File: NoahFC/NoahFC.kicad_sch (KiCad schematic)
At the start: 30 parts, among them J1 ALERON, J10 GND, J11 SCK, J12 MISO, J13 VCC, J14 GND, J2 ELEVATOR, J3 MPU6050, J4 FTDI, J5 VCC, J6 THROTTLE, J7 PPM, J8 GPS, U1 ATmega328, U3 AMS1117-5.0, Y1 16Mhz

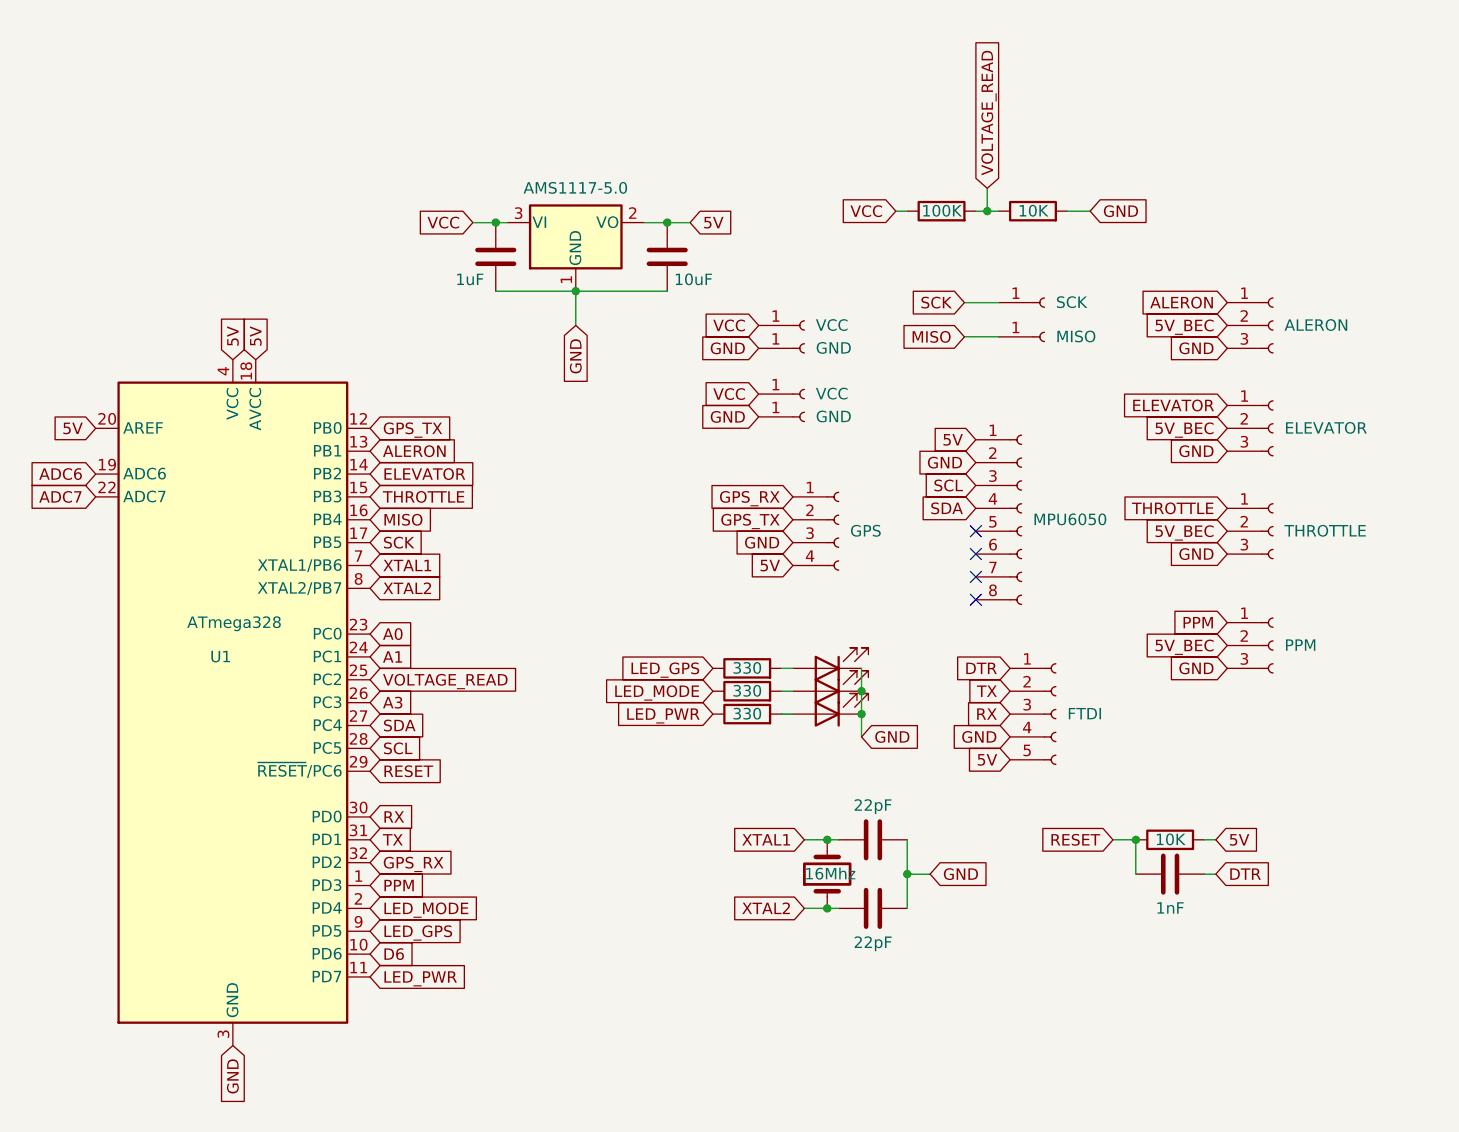
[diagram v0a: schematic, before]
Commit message: route board
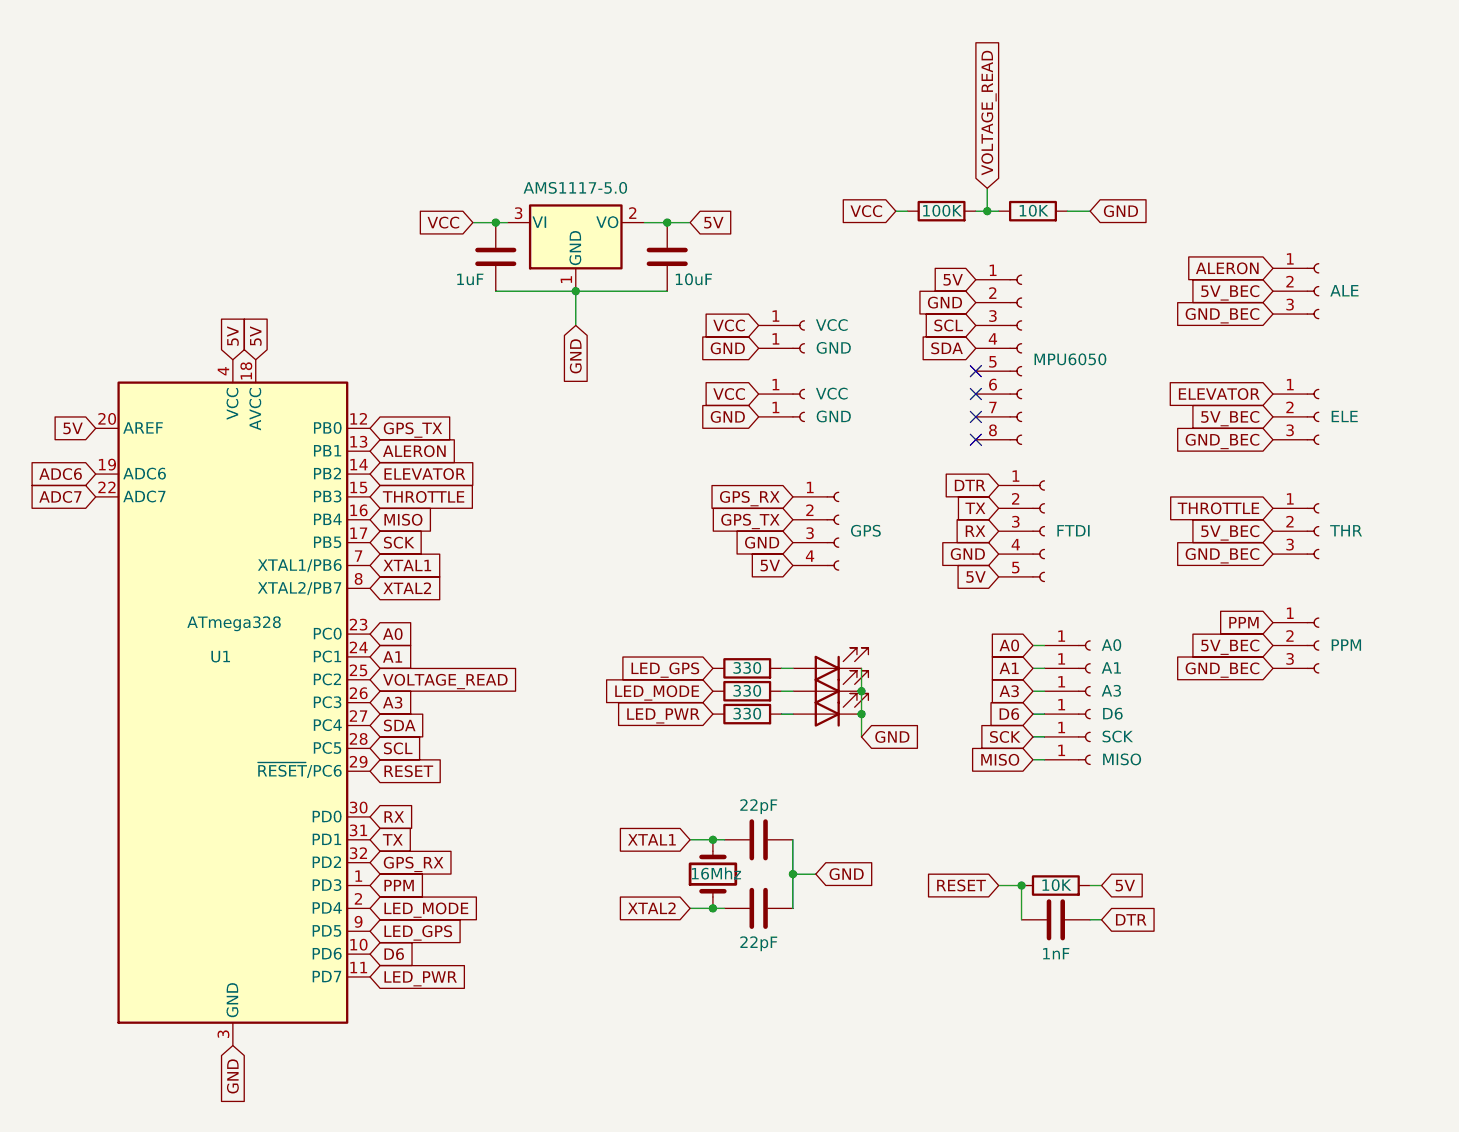
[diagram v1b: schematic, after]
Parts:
- added J15: A1, TestPoint:TestPoint_Pad_1.0x1.0mm, symbol Connector:Conn_01x01_Female
- added J16: A3, TestPoint:TestPoint_Pad_1.0x1.0mm, symbol Connector:Conn_01x01_Female
- added J17: D6, TestPoint:TestPoint_Pad_1.0x1.0mm, symbol Connector:Conn_01x01_Female
- added J9: A0, TestPoint:TestPoint_Pad_1.0x1.0mm, symbol Connector:Conn_01x01_Female
- J1: value ALERON -> ALE
- J2: value ELEVATOR -> ELE
- J6: value THROTTLE -> THR
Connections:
- net A0: now also J9.1 (Pin_1)
- net A1: now also J15.1 (Pin_1)
- net A3: now also J16.1 (Pin_1)
- net D6: now also J17.1 (Pin_1)
- net GND: no longer J1.3 (Pin_3), J2.3 (Pin_3), J6.3 (Pin_3), J7.3 (Pin_3)
- new net GND_BEC: J1.3 (Pin_3), J2.3 (Pin_3), J6.3 (Pin_3), J7.3 (Pin_3)

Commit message: rev1 updates
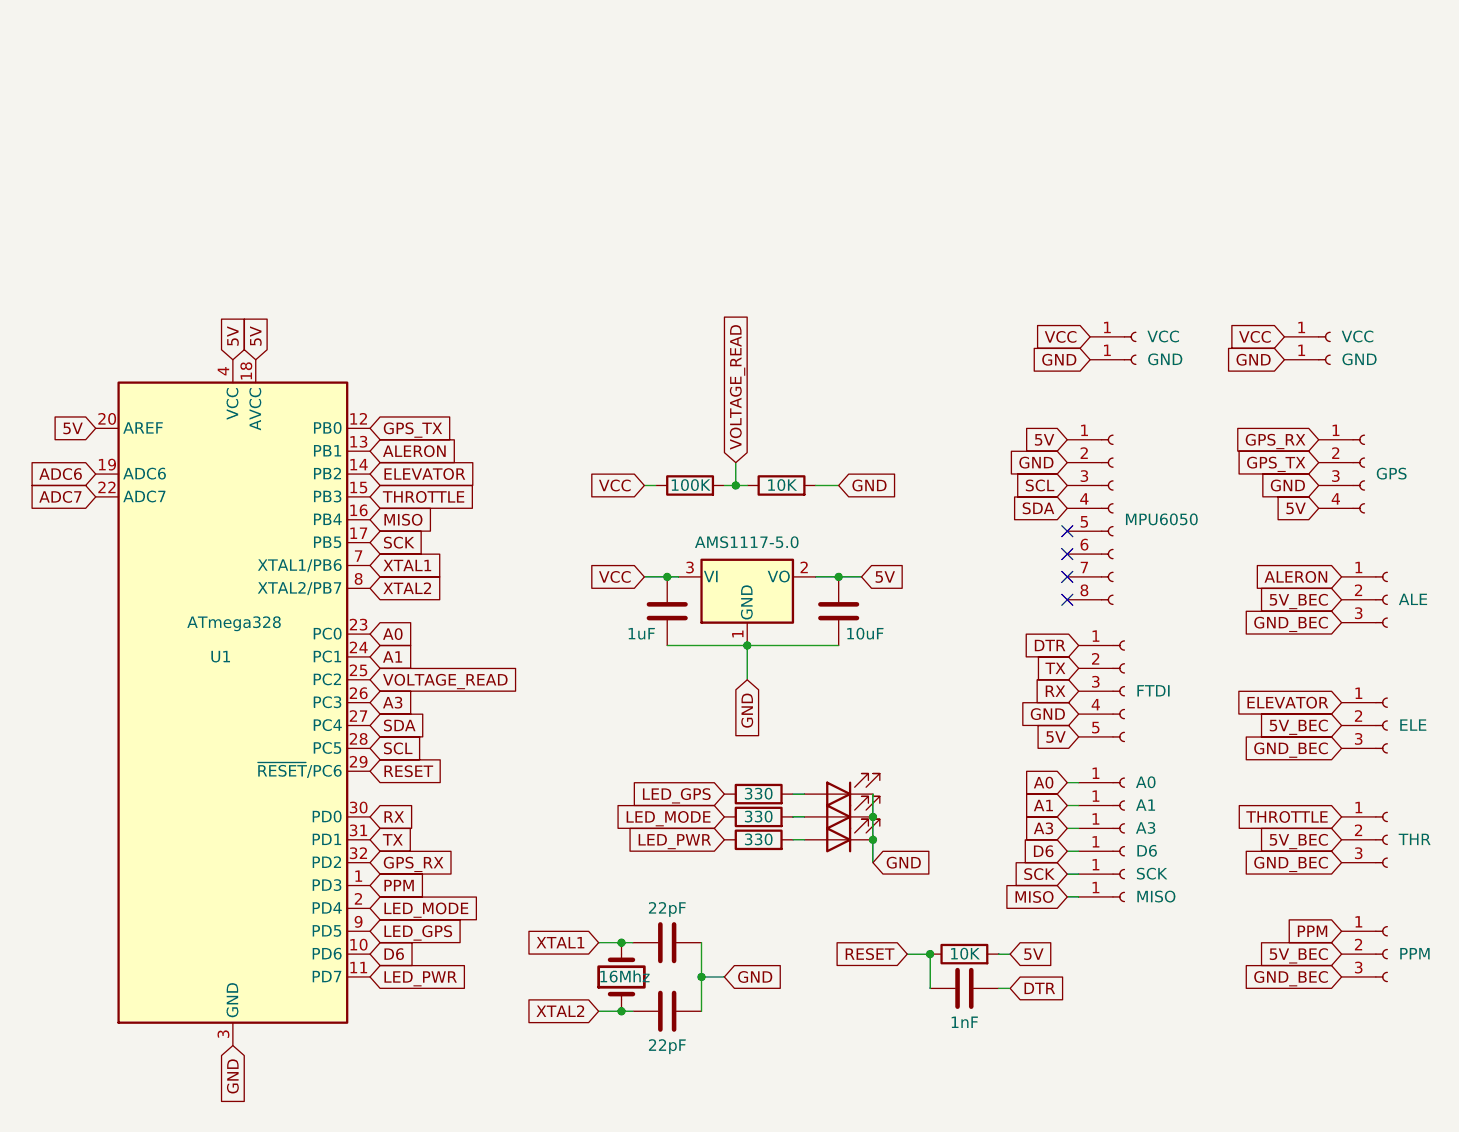
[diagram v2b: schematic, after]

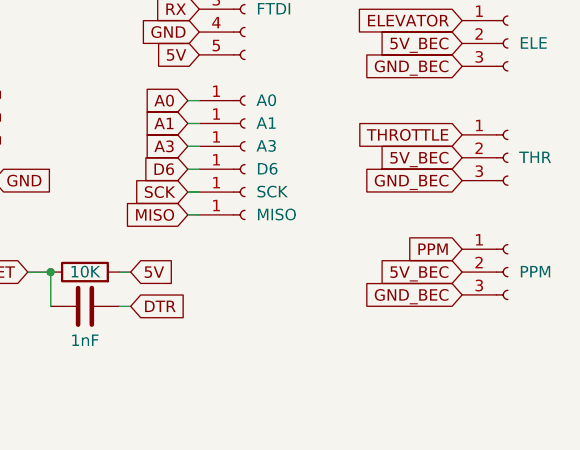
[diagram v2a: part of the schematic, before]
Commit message: pin improve
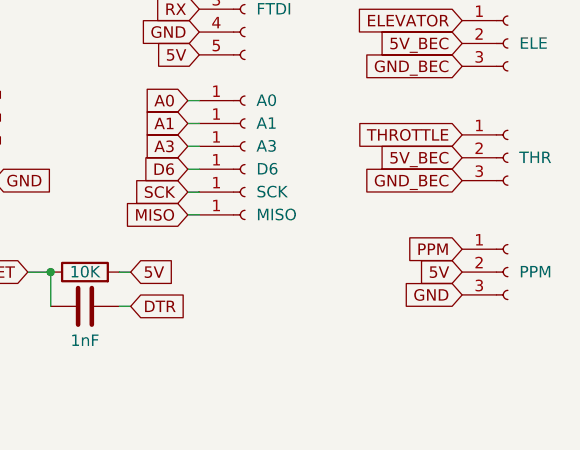
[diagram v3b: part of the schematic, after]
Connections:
- net 5V: now also J7.2 (Pin_2)
- net 5V_BEC: no longer J7.2 (Pin_2)
- net GND: now also J7.3 (Pin_3)
- net GND_BEC: no longer J7.3 (Pin_3)
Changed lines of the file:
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@@
     )
   )
-  (global_label "5V_BEC" (shape input) (at 222.25 124.46 180) (fields_autoplaced)
+  (global_label "5V" (shape input) (at 222.25 124.46 180) (fields_autoplaced)
     (effects (font (size 1.27 1.27)) (justify right))
-    (property "Intersheet References" "${INTERSHEET_REFS}" (id 0) (at 212.8821 124.3806 0)
+    (property "Intersheet References" "${INTERSHEET_REFS}" (id 0) (at 217.5388 124.3806 0)
       (effects (font (size 1.27 1.27)) (justify right) hide)
     )
@@
     )
   )
-  (global_label "GND_BEC" (shape input) (at 222.25 127 180) (fields_autoplaced)
+  (global_label "GND" (shape input) (at 222.25 127 180) (fields_autoplaced)
     (effects (font (size 1.27 1.27)) (justify right))
-    (property "Intersheet References" "${INTERSHEET_REFS}" (id 0) (at 211.3098 126.9206 0)
+    (property "Intersheet References" "${INTERSHEET_REFS}" (id 0) (at 215.9664 126.9206 0)
       (effects (font (size 1.27 1.27)) (justify right) hide)
     )
